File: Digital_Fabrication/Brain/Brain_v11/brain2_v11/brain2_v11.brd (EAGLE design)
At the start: 140.7 x 108 mm, 90 parts, among them J6 ELECTRO_MECH_PAD, J7 ELECTRO_MECH_PAD, J8 ELECTRO_MECH_PAD, J9 ELECTRO_MECH_PAD

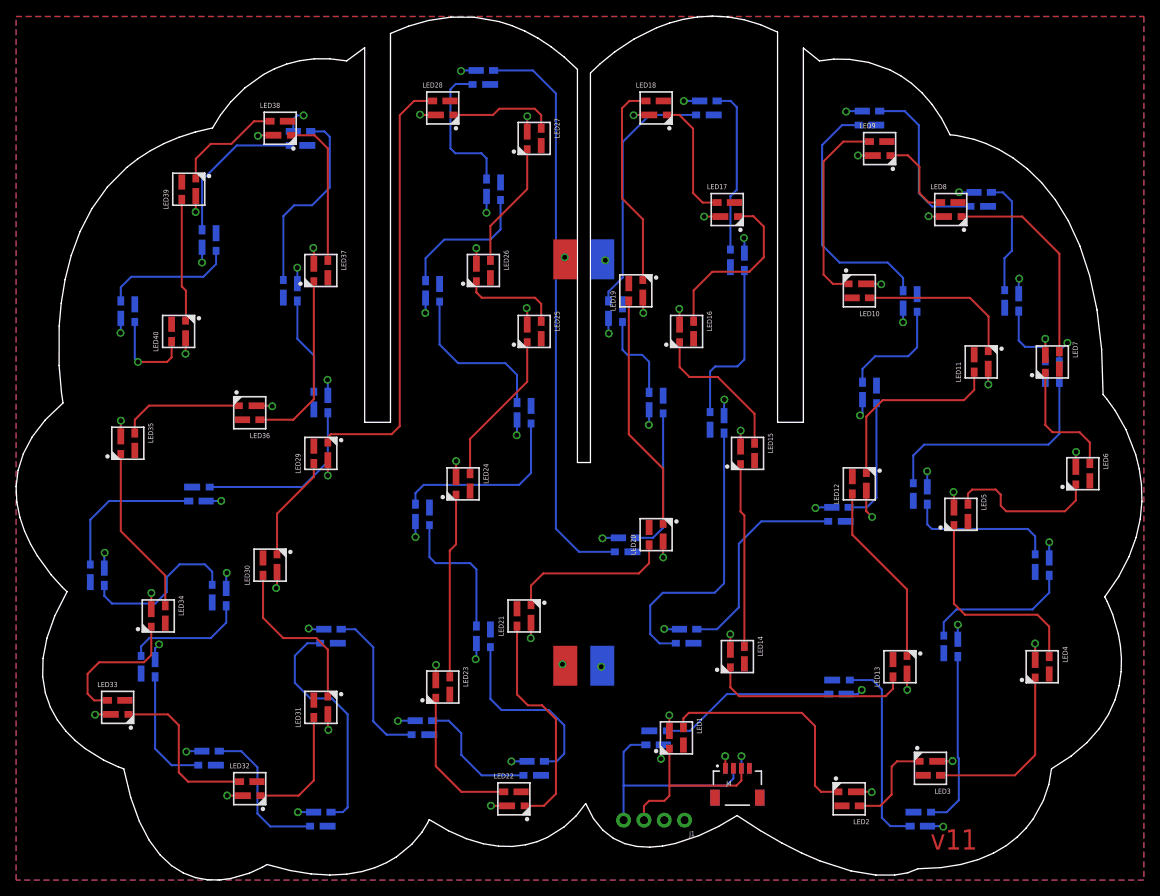
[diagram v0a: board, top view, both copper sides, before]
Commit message: brain boards v11
Added custom silkscreen
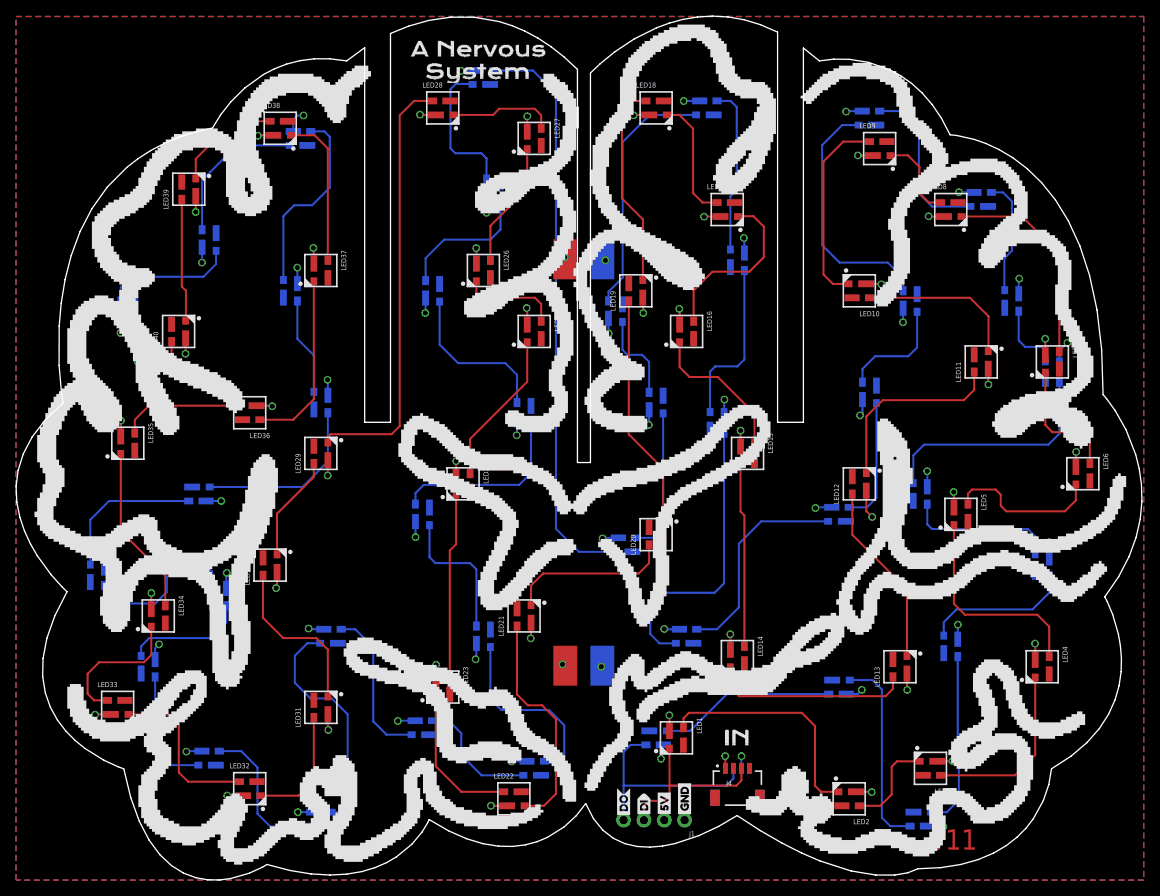
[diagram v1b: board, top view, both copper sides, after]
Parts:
- added U$1: A_NERVOUS0, brain:A_NERVOUS0
- added U$10, U$11: DO3, brain:DO3
- added U$12: IN0, brain:IN0
- added U$13: OUT1, brain:OUT1
- added U$14: BRAIN2_PCB_TOP_SILK, brain:BRAIN2_PCB_TOP_SILK
- added U$15: BRAIN2_PCB_BOT_SILK, brain:BRAIN2_PCB_BOT_SILK
- added U$2: SYSTEM1, brain:SYSTEM1
- added U$3: MAKIN_STUFF2, brain:MAKIN_STUFF2
- added U$4, U$5: 5V1, brain:5V1
- added U$6, U$7: GND0, brain:GND0
- added U$8, U$9: DI0, brain:DI0
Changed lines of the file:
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@@
 <?xml version="1.0" encoding="utf-8"?>
 <!DOCTYPE eagle SYSTEM "eagle.dtd">
-<eagle version="9.5.2">
+<eagle version="9.6.2">
 <drawing>
 <settings>
-<setting alwaysvectorfont="no"/>
+<setting alwaysvectorfont="yes"/>
 <setting verticaltext="up"/>
 </settings>
@@
 <layer number="37" name="tTest" color="7" fill="1" visible="no" active="yes"/>
 <layer number="38" name="bTest" color="7" fill="1" visible="no" active="yes"/>
-<layer number="39" name="tKeepout" color="4" fill="11" visible="yes" active="yes"/>
-<layer number="40" name="bKeepout" color="1" fill="11" visible="yes" active="yes"/>
+<layer number="39" name="tKeepout" color="4" fill="11" visible="no" active="yes"/>
+<layer number="40" name="bKeepout" color="1" fill="11" visible="no" active="yes"/>
 <layer number="41" name="tRestrict" color="4" fill="10" visible="no" active="yes"/>
 <layer number="42" name="bRestrict" color="1" fill="10" visible="no" active="yes"/>
@@
 <layer number="44" name="Drills" color="7" fill="1" visible="no" active="yes"/>
 <layer number="45" name="Holes" color="7" fill="1" visible="yes" active="yes"/>
-<layer number="46" name="Milling" color="3" fill="1" visible="no" active="yes"/>
+<layer number="46" name="Milling" color="3" fill="1" visible="yes" active="yes"/>
 <layer number="47" name="Measures" color="7" fill="1" visible="no" active="yes"/>
 <layer number="48" name="Document" color="7" fill="1" visible="no" active="yes"/>
@@
 <element name="J8" library="brain" package="5X3_SOLDER_PAD" value="ELECTRO_MECH_PAD" x="73.279" y="77.59525" smashed="yes" rot="MR270"/>
 <element name="J9" library="brain" package="5X3_SOLDER_PAD" value="ELECTRO_MECH_PAD" x="73.279" y="26.79525" smashed="yes" rot="MR270"/>
+<element name="U$1" library="brain" package="A_NERVOUS0" value="A_NERVOUS0" x="47.752" y="103.886" smashed="yes"/>
+<element name="U$2" library="brain" package="SYSTEM1" value="SYSTEM1" x="49.53" y="101.092" smashed="yes"/>
+<element name="U$3" library="brain" package="MAKIN_STUFF2" value="MAKIN_STUFF2" x="37.211" y="6.604" smashed="yes" rot="MR0"/>
+<element name="U$4" library="brain" package="5V1" value="5V1" x="81.026" y="7.747" smashed="yes" rot="R90"/>
+<element name="U$5" library="brain" package="5V1" value="5V1" x="81.026" y="7.747" smashed="yes" rot="MR90"/>
+<element name="U$6" library="brain" package="GND0" value="GND0" x="83.566" y="7.747" smashed="yes" rot="R90"/>
+<element name="U$7" library="brain" package="GND0" value="GND0" x="83.566" y="7.747" smashed="yes" rot="MR90"/>
+<element name="U$8" library="brain" package="DI0" value="DI0" x="78.486" y="7.747" smashed="yes" rot="R90"/>
+<element name="U$9" library="brain" package="DI0" value="DI0" x="78.486" y="7.747" smashed="yes" rot="MR90"/>
+<element name="U$10" library="brain" package="DO3" value="DO3" x="75.946" y="7.62" smashed="yes" rot="R90"/>
+<element name="U$11" library="brain" package="DO3" value="DO3" x="75.946" y="7.62" smashed="yes" rot="MR90"/>
+<element name="U$12" library="brain" package="IN0" value="IN0" x="86.868" y="17.78" smashed="yes"/>
+<element name="U$13" library="brain" package="OUT1" value="OUT1" x="95.123" y="17.78" smashed="yes" rot="MR0"/>
+<element name="U$14" library="brain" package="BRAIN2_PCB_TOP_SILK" value="BRAIN2_PCB_TOP_SILK" x="69.85" y="54.61" smashed="yes"/>
+<element name="U$15" library="brain" package="BRAIN2_PCB_BOT_SILK" value="BRAIN2_PCB_BOT_SILK" x="70.358" y="54.229" smashed="yes" rot="MR0"/>
 </elements>
 <signals>
